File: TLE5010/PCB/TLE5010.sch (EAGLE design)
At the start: 10 parts, among them J2 22-27-2061-06, U1 TLE5010

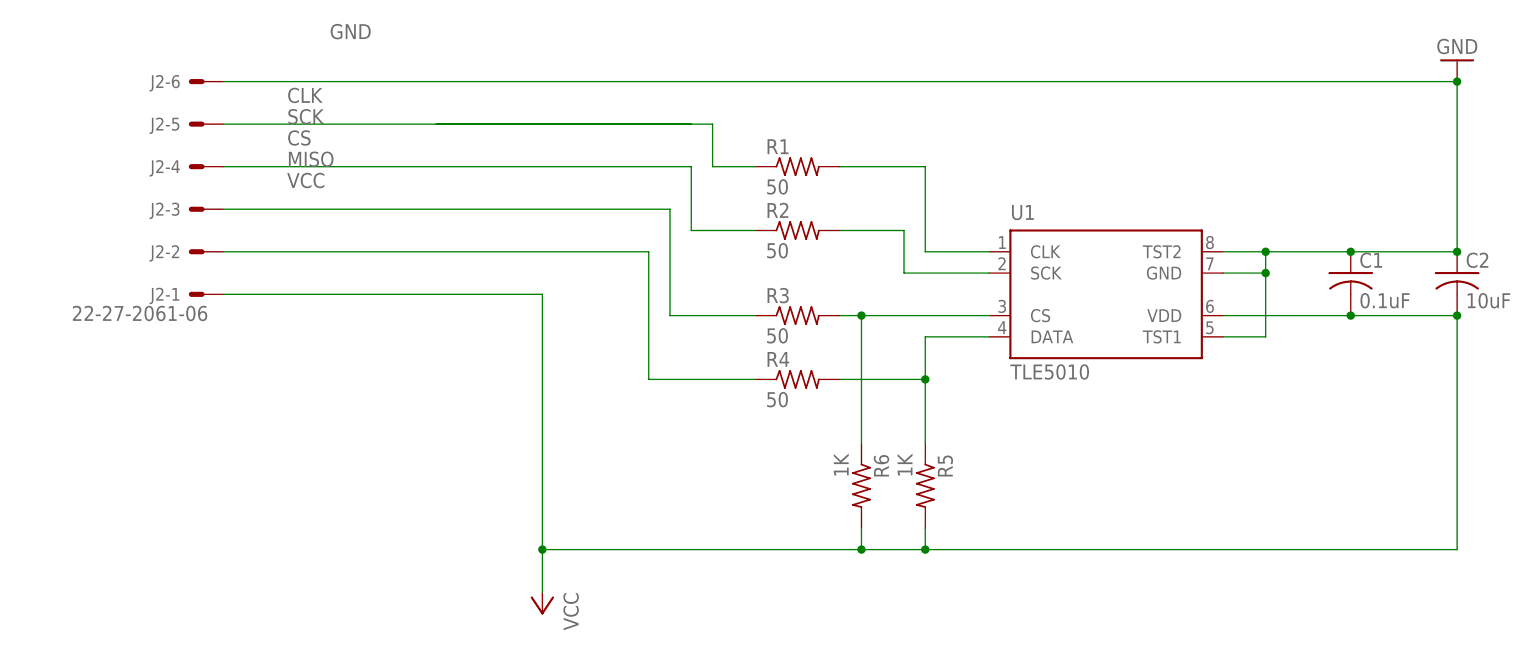
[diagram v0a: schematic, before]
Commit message: TLE5010.brd fixed
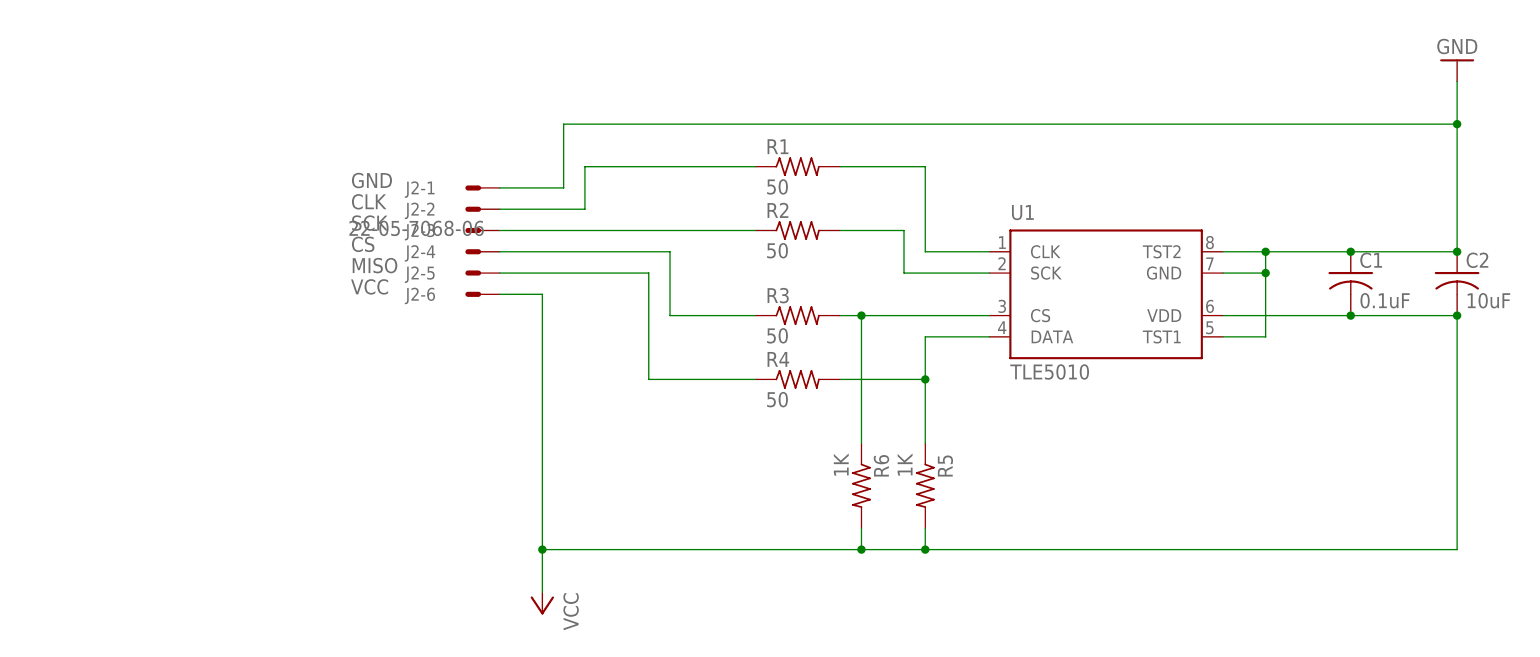
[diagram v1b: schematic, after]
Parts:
- J2: value 22-27-2061-06 -> 22-05-7068-06; device con-molex:22-27-2061-06 -> con-molex:22-05-7068-06
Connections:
- net CLK: now also J2-2.S; no longer J2-5.S
- net CS: now also J2-4.S; no longer J2-3.S
- net GND: now also J2-1.S; no longer J2-6.S
- net MISO: now also J2-5.S; no longer J2-2.S
- net SCK: now also J2-3.S; no longer J2-4.S
- net VCC: now also J2-6.S; no longer J2-1.S
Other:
- moved on the sheet: J2-1, J2-2, J2-3, J2-4, J2-5, J2-6
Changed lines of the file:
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@@
 <part name="P+2" library="supply1" deviceset="VCC" device=""/>
 <part name="GND2" library="supply1" deviceset="GND" device=""/>
-<part name="J2" library="con-molex" library_urn="urn:adsk.eagle:library:165" deviceset="22-?-06" device="27-2061" package3d_urn="urn:adsk.eagle:package:8078653/1"/>
+<part name="J2" library="con-molex" library_urn="urn:adsk.eagle:library:165" deviceset="22-?-06" device="05-7068" package3d_urn="urn:adsk.eagle:package:8078652/1" value="22-05-7068-06"/>
 </parts>
 <sheets>
@@
 <attribute name="VALUE" x="93.98" y="76.2" size="1.778" layer="96" rot="R180"/>
 </instance>
-<instance part="J2" gate="-1" x="-58.42" y="45.72" smashed="yes" rot="R180">
-<attribute name="NAME" x="-60.96" y="46.482" size="1.524" layer="95" rot="R180"/>
-<attribute name="VALUE" x="-57.658" y="44.323" size="1.778" layer="96" rot="R180"/>
-</instance>
-<instance part="J2" gate="-2" x="-58.42" y="50.8" smashed="yes" rot="R180">
-<attribute name="NAME" x="-60.96" y="51.562" size="1.524" layer="95" rot="R180"/>
-</instance>
-<instance part="J2" gate="-3" x="-58.42" y="55.88" smashed="yes" rot="R180">
-<attribute name="NAME" x="-60.96" y="56.642" size="1.524" layer="95" rot="R180"/>
-</instance>
-<instance part="J2" gate="-4" x="-58.42" y="60.96" smashed="yes" rot="R180">
-<attribute name="NAME" x="-60.96" y="61.722" size="1.524" layer="95" rot="R180"/>
-</instance>
-<instance part="J2" gate="-5" x="-58.42" y="66.04" smashed="yes" rot="R180">
-<attribute name="NAME" x="-60.96" y="66.802" size="1.524" layer="95" rot="R180"/>
-</instance>
-<instance part="J2" gate="-6" x="-58.42" y="71.12" smashed="yes" rot="R180">
-<attribute name="NAME" x="-60.96" y="71.882" size="1.524" layer="95" rot="R180"/>
+<instance part="J2" gate="-1" x="-25.4" y="58.42" smashed="yes" rot="R180">
+<attribute name="NAME" x="-30.48" y="59.182" size="1.524" layer="95" rot="R180"/>
+<attribute name="VALUE" x="-24.638" y="54.483" size="1.778" layer="96" rot="R180"/>
+</instance>
+<instance part="J2" gate="-2" x="-25.4" y="55.88" smashed="yes" rot="R180">
+<attribute name="NAME" x="-30.48" y="56.642" size="1.524" layer="95" rot="R180"/>
+</instance>
+<instance part="J2" gate="-3" x="-25.4" y="53.34" smashed="yes" rot="R180">
+<attribute name="NAME" x="-30.48" y="54.102" size="1.524" layer="95" rot="R180"/>
+</instance>
+<instance part="J2" gate="-4" x="-25.4" y="50.8" smashed="yes" rot="R180">
+<attribute name="NAME" x="-30.48" y="51.562" size="1.524" layer="95" rot="R180"/>
+</instance>
+<instance part="J2" gate="-5" x="-25.4" y="48.26" smashed="yes" rot="R180">
+<attribute name="NAME" x="-30.48" y="49.022" size="1.524" layer="95" rot="R180"/>
+</instance>
+<instance part="J2" gate="-6" x="-25.4" y="45.72" smashed="yes" rot="R180">
+<attribute name="NAME" x="-30.48" y="46.482" size="1.524" layer="95" rot="R180"/>
 </instance>
 </instances>
@@
 <net name="CS" class="0">
 <segment>
-<wire x1="-2.54" y1="43.18" x2="-2.54" y2="55.88" width="0.1524" layer="91"/>
+<wire x1="-2.54" y1="43.18" x2="-2.54" y2="50.8" width="0.1524" layer="91"/>
 <pinref part="R3" gate="G$1" pin="1"/>
 <wire x1="7.62" y1="43.18" x2="-2.54" y2="43.18" width="0.1524" layer="91"/>
-<label x="-48.26" y="63.5" size="1.778" layer="95"/>
+<label x="-40.64" y="50.8" size="1.778" layer="95"/>
+<pinref part="J2" gate="-4" pin="S"/>
+<wire x1="-22.86" y1="50.8" x2="-2.54" y2="50.8" width="0.1524" layer="91"/>
+</segment>
+</net>
+<net name="SCK" class="0">
+<segment>
+<pinref part="R2" gate="G$1" pin="1"/>
+<label x="-40.64" y="53.34" size="1.778" layer="95"/>
 <pinref part="J2" gate="-3" pin="S"/>
-<wire x1="-55.88" y1="55.88" x2="-2.54" y2="55.88" width="0.1524" layer="91"/>
-</segment>
-</net>
-<net name="SCK" class="0">
-<segment>
-<pinref part="R2" gate="G$1" pin="1"/>
-<wire x1="0" y1="60.96" x2="0" y2="53.34" width="0.1524" layer="91"/>
-<wire x1="0" y1="53.34" x2="7.62" y2="53.34" width="0.1524" layer="91"/>
-<label x="-48.26" y="66.04" size="1.778" layer="95"/>
-<pinref part="J2" gate="-4" pin="S"/>
-<wire x1="-55.88" y1="60.96" x2="0" y2="60.96" width="0.1524" layer="91"/>
+<wire x1="-22.86" y1="53.34" x2="7.62" y2="53.34" width="0.1524" layer="91"/>
 </segment>
 </net>
@@
 <junction x="27.94" y="15.24"/>
 <junction x="-17.78" y="15.24"/>
-<label x="-48.26" y="58.42" size="1.778" layer="95"/>
+<label x="-40.64" y="45.72" size="1.778" layer="95"/>
 <wire x1="-17.78" y1="45.72" x2="-17.78" y2="15.24" width="0.1524" layer="91"/>
-<pinref part="J2" gate="-1" pin="S"/>
-<wire x1="-55.88" y1="45.72" x2="-17.78" y2="45.72" width="0.1524" layer="91"/>
+<pinref part="J2" gate="-6" pin="S"/>
+<wire x1="-22.86" y1="45.72" x2="-17.78" y2="45.72" width="0.1524" layer="91"/>
 </segment>
 </net>
@@
 <segment>
 <pinref part="R4" gate="G$1" pin="1"/>
-<wire x1="-5.08" y1="50.8" x2="-5.08" y2="35.56" width="0.1524" layer="91"/>
+<wire x1="-5.08" y1="48.26" x2="-5.08" y2="35.56" width="0.1524" layer="91"/>
 <wire x1="-5.08" y1="35.56" x2="7.62" y2="35.56" width="0.1524" layer="91"/>
-<label x="-48.26" y="60.96" size="1.778" layer="95"/>
-<pinref part="J2" gate="-2" pin="S"/>
-<wire x1="-55.88" y1="50.8" x2="-5.08" y2="50.8" width="0.1524" layer="91"/>
+<label x="-40.64" y="48.26" size="1.778" layer="95"/>
+<pinref part="J2" gate="-5" pin="S"/>
+<wire x1="-22.86" y1="48.26" x2="-5.08" y2="48.26" width="0.1524" layer="91"/>
 </segment>
 </net>
@@
 <pinref part="C1" gate="G$1" pin="1"/>
 <wire x1="78.74" y1="50.8" x2="91.44" y2="50.8" width="0.1524" layer="91"/>
-<wire x1="91.44" y1="71.12" x2="91.44" y2="50.8" width="0.1524" layer="91"/>
+<wire x1="91.44" y1="71.12" x2="91.44" y2="66.04" width="0.1524" layer="91"/>
 <junction x="91.44" y="50.8"/>
 <pinref part="GND2" gate="1" pin="GND"/>
 <pinref part="U1" gate="G$1" pin="TST2"/>
+<wire x1="91.44" y1="66.04" x2="91.44" y2="50.8" width="0.1524" layer="91"/>
 <wire x1="63.5" y1="50.8" x2="68.58" y2="50.8" width="0.1524" layer="91"/>
 <junction x="78.74" y="50.8"/>
@@
 <wire x1="63.5" y1="48.26" x2="68.58" y2="48.26" width="0.1524" layer="91"/>
 <junction x="68.58" y="48.26"/>
-<label x="-43.18" y="76.2" size="1.778" layer="95"/>
-<wire x1="-55.88" y1="71.12" x2="91.44" y2="71.12" width="0.1524" layer="91"/>
-<junction x="91.44" y="71.12"/>
-<pinref part="J2" gate="-6" pin="S"/>
+<label x="-40.64" y="58.42" size="1.778" layer="95"/>
+<pinref part="J2" gate="-1" pin="S"/>
+<wire x1="-22.86" y1="58.42" x2="-15.24" y2="58.42" width="0.1524" layer="91"/>
+<wire x1="-15.24" y1="58.42" x2="-15.24" y2="66.04" width="0.1524" layer="91"/>
+<wire x1="-15.24" y1="66.04" x2="91.44" y2="66.04" width="0.1524" layer="91"/>
+<junction x="91.44" y="66.04"/>
 </segment>
 </net>
@@
 <segment>
 <pinref part="R1" gate="G$1" pin="1"/>
-<wire x1="2.54" y1="60.96" x2="7.62" y2="60.96" width="0.1524" layer="91"/>
-<label x="-48.26" y="68.58" size="1.778" layer="95"/>
-<wire x1="2.54" y1="66.04" x2="2.54" y2="60.96" width="0.1524" layer="91"/>
-<pinref part="J2" gate="-5" pin="S"/>
-<wire x1="-55.88" y1="66.04" x2="2.54" y2="66.04" width="0.1524" layer="91"/>
+<label x="-40.64" y="55.88" size="1.778" layer="95"/>
+<pinref part="J2" gate="-2" pin="S"/>
+<wire x1="-22.86" y1="55.88" x2="-12.7" y2="55.88" width="0.1524" layer="91"/>
+<wire x1="-12.7" y1="55.88" x2="-12.7" y2="60.96" width="0.1524" layer="91"/>
+<wire x1="-12.7" y1="60.96" x2="7.62" y2="60.96" width="0.1524" layer="91"/>
 </segment>
 </net>
@@
 </segment>
 </net>
-<net name="N$4" class="0">
-<segment>
-<wire x1="0" y1="66.04" x2="-30.48" y2="66.04" width="0.1524" layer="91"/>
-</segment>
-</net>
